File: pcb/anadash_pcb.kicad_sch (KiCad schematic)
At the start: 23 parts, among them J1 Meter1, J2 Meter2, J3 Meter3, J4 Meter4, SW1 SW_Push, SW2 SW_Push, SW3 SW_Push, SW4 SW_Push, SW5 SW_Push, SW6 SW_Push, SW7 SW_Push, SW8 SW_Push, U2 ER_OLEDM0.91_1x-I2C

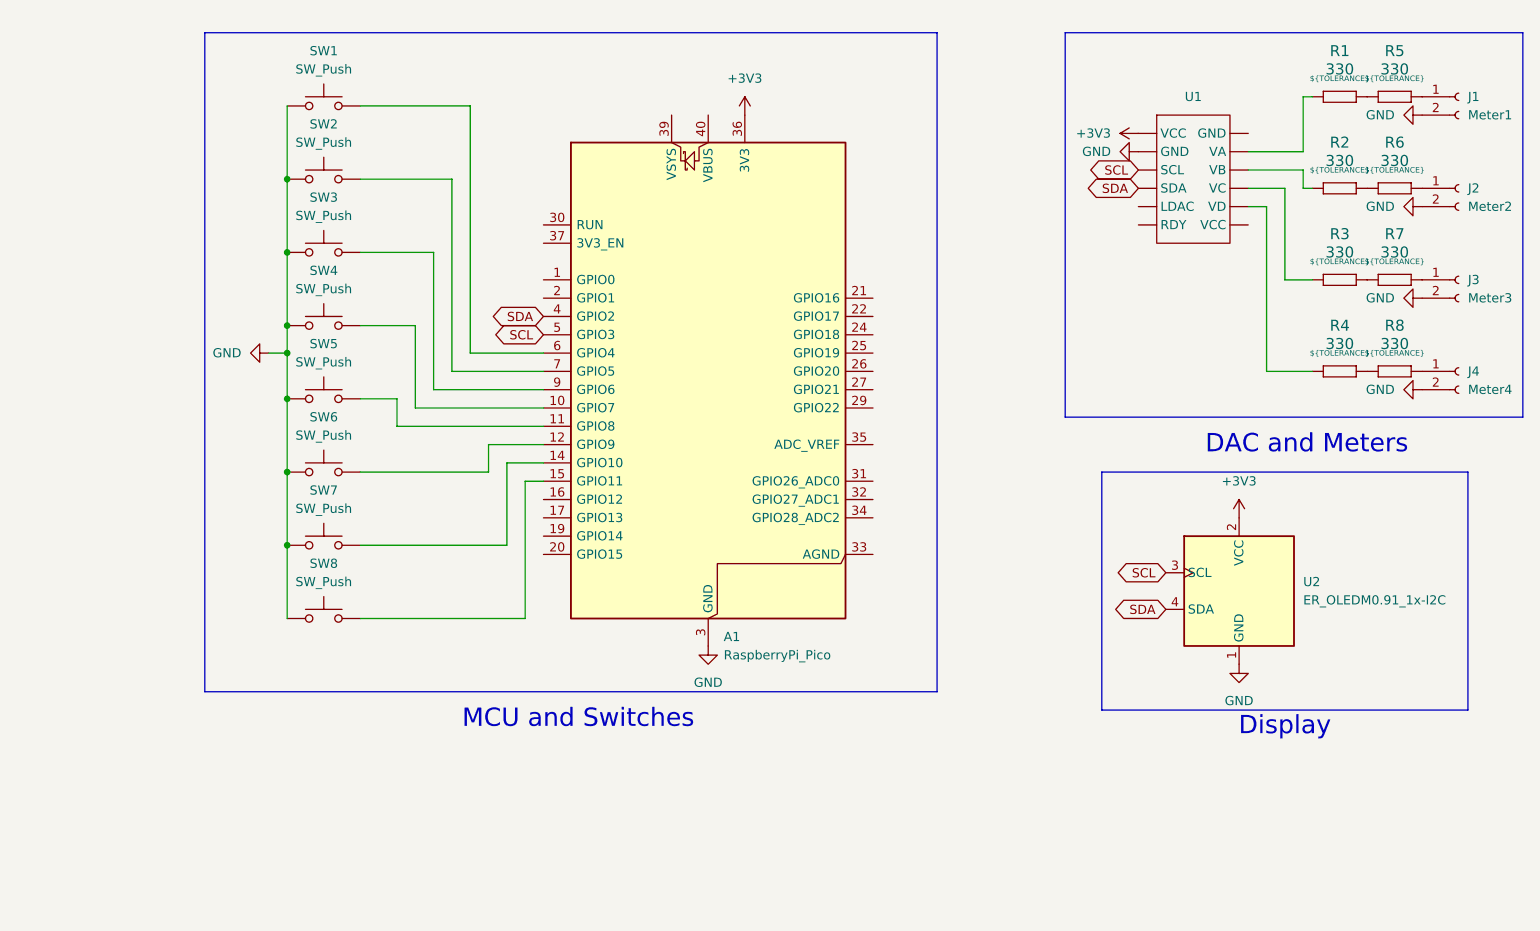
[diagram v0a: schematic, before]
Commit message: esp32 switch :d
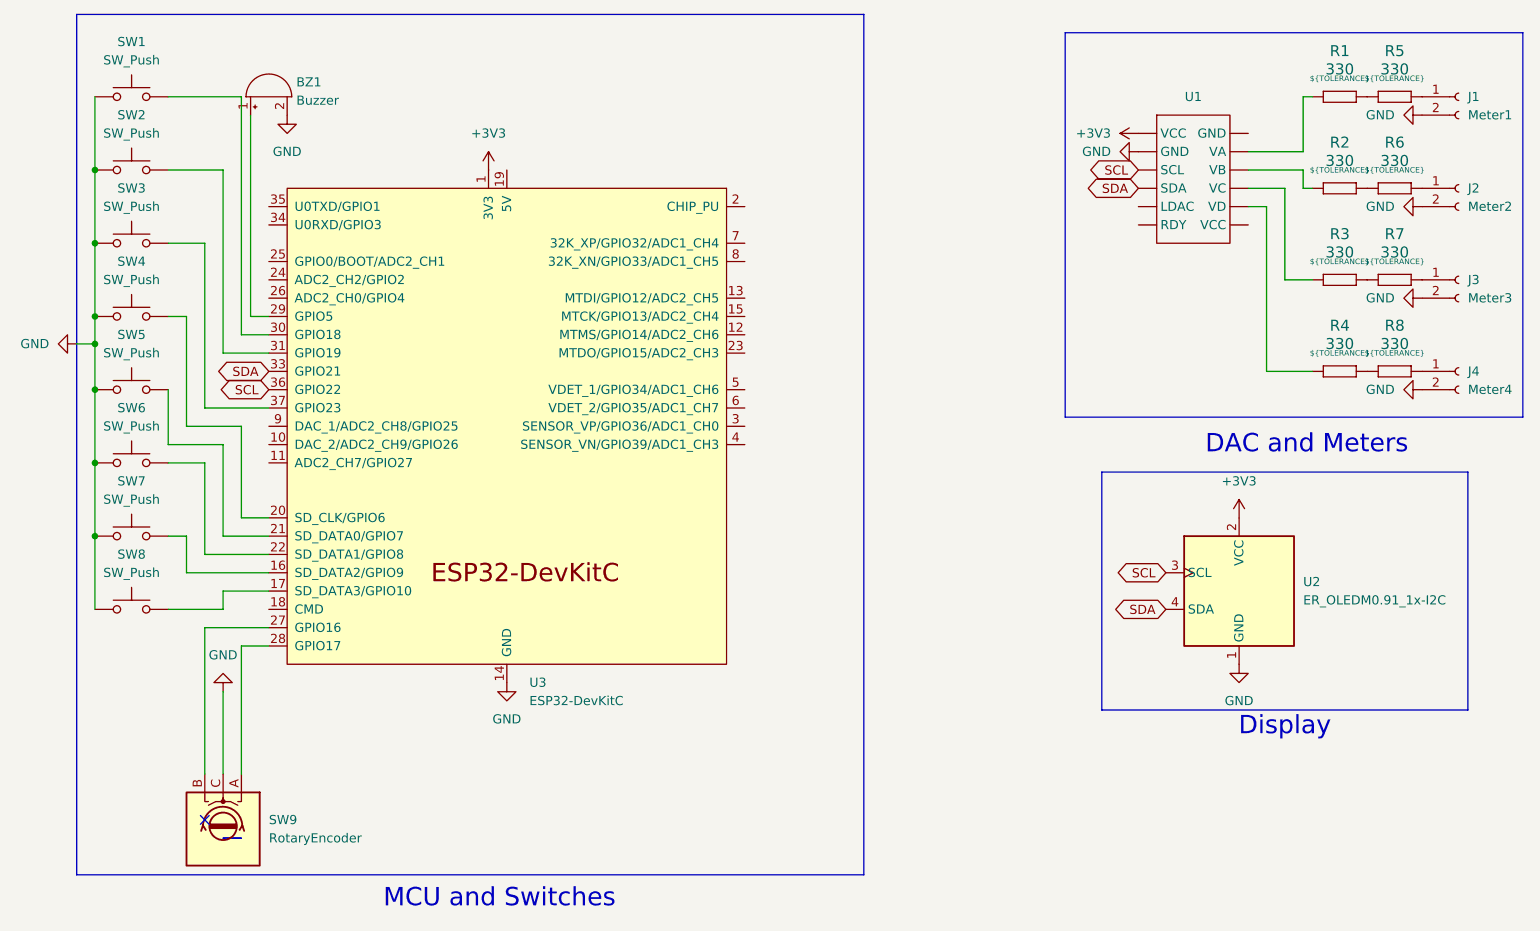
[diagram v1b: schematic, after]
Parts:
- removed A1: RaspberryPi_Pico, Module:RaspberryPi_Pico_Common_Unspecified, symbol MCU_Module:RaspberryPi_Pico
- added BZ1: Buzzer, Buzzer_Beeper:Buzzer_D14mm_H7mm_P10mm, symbol Device:Buzzer
- added SW9: RotaryEncoder, symbol Device:RotaryEncoder
- added U3: ESP32-DevKitC, PCM_Espressif:ESP32-DevKitC, symbol Espressif:ESP32-DevKitC
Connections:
- net +3V3: now also U3.1 (3V3)
- net GND: now also BZ1.2 (-), SW9.C, U3.14 (GND), U3.32 (GND), U3.38 (GND)
- net SCL: now also U3.36 (GPIO22)
- net SDA: now also U3.33 (GPIO21)
- net at SW4.2: now also U3.20 (SD_CLK/GPIO6)
- net at SW5.2: now also U3.21 (SD_DATA0/GPIO7)
- net at SW6.2: now also U3.22 (SD_DATA1/GPIO8)
- net at SW7.2: now also U3.16 (SD_DATA2/GPIO9)
- net at SW8.2: now also U3.17 (SD_DATA3/GPIO10)
- net at SW1.2: now also U3.30 (GPIO18)
- net at SW2.2: now also U3.31 (GPIO19)
- net at SW3.2: now also U3.37 (GPIO23)
- new net: SW9.B, U3.27 (GPIO16)
- new net: SW9.A, U3.28 (GPIO17)
- new net: BZ1.1 (+), U3.29 (GPIO5)
- no-connect marks 0 -> 1
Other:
- title: (none) -> Anadash PCB
- moved on the sheet: SW1, SW2, SW3, SW4, SW5, SW6, SW7, SW8
